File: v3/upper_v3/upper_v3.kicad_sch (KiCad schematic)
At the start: 3 parts, among them J1 Conn_01x18, J2 Conn_01x09_Male, J3 Conn_01x09_Male

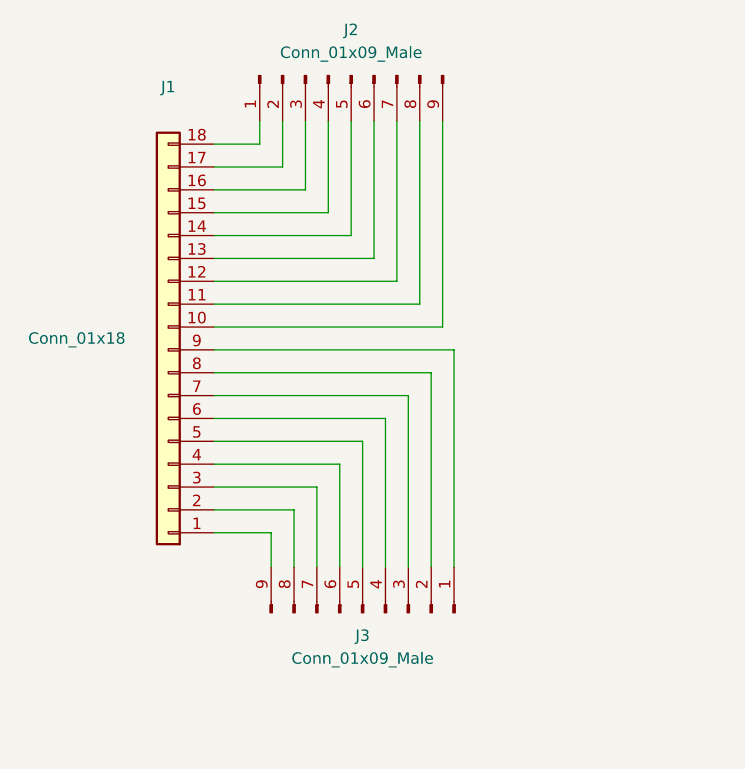
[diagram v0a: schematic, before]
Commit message: Complete Toast PCB
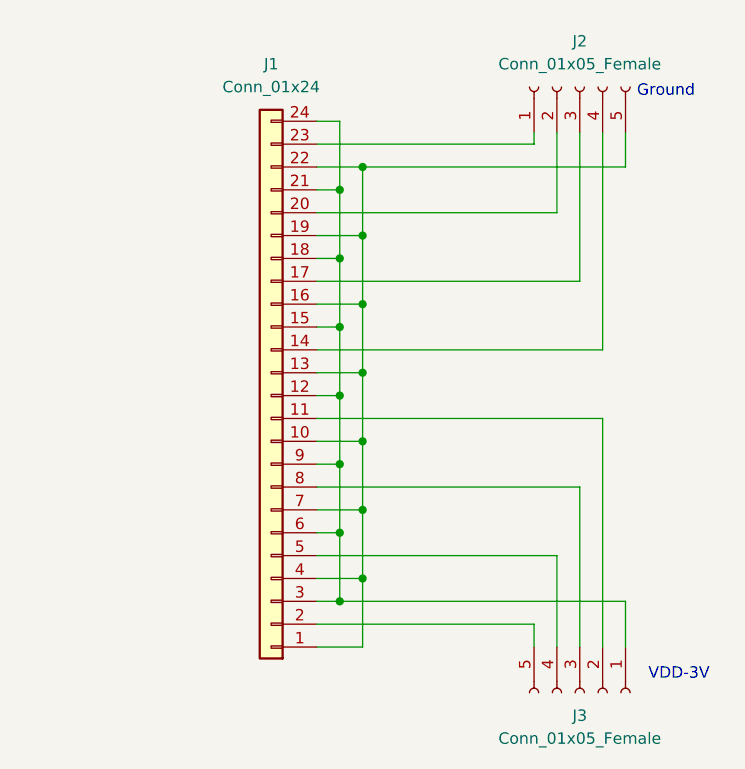
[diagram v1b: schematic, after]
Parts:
- removed J1: Conn_01x18, Connector_PinHeader_2.54mm:PinHeader_1x18_P2.54mm_Horizontal, symbol Connector_Generic:Conn_01x18
- removed J2, J3: Conn_01x09_Male, Connector_PinSocket_2.54mm:PinSocket_1x09_P2.54mm_Vertical, symbol Connector:Conn_01x09_Male
- added J1: Conn_01x24, Connector_PinHeader_2.54mm:PinHeader_1x24_P2.54mm_Horizontal, symbol Connector_Generic:Conn_01x24
- added J2, J3: Conn_01x05_Female, Connector_PinSocket_2.54mm:PinSocket_1x05_P2.54mm_Vertical, symbol Connector:Conn_01x05_Female
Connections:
- new net: J1.23 (Pin_23), J2.1 (Pin_1)
- new net: J1.20 (Pin_20), J2.2 (Pin_2)
- new net: J1.17 (Pin_17), J2.3 (Pin_3)
- new net: J1.14 (Pin_14), J2.4 (Pin_4)
- new net: J1.1 (Pin_1), J1.10 (Pin_10), J1.13 (Pin_13), J1.16 (Pin_16), J1.19 (Pin_19), J1.22 (Pin_22), J1.4 (Pin_4), J1.7 (Pin_7), J2.5 (Pin_5)
- new net: J1.11 (Pin_11), J3.2 (Pin_2)
- new net: J1.12 (Pin_12), J1.15 (Pin_15), J1.18 (Pin_18), J1.21 (Pin_21), J1.24 (Pin_24), J1.3 (Pin_3), J1.6 (Pin_6), J1.9 (Pin_9), J3.1 (Pin_1)
- new net: J1.2 (Pin_2), J3.5 (Pin_5)
- new net: J1.5 (Pin_5), J3.4 (Pin_4)
- new net: J1.8 (Pin_8), J3.3 (Pin_3)
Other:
- note added: "Ground"
- note added: "VDD-3V"
